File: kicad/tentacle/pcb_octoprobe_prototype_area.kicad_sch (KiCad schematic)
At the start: 15 parts, among them J1301 Conn_01x20, J1302 Conn_01x20, J1303 Conn_01x20

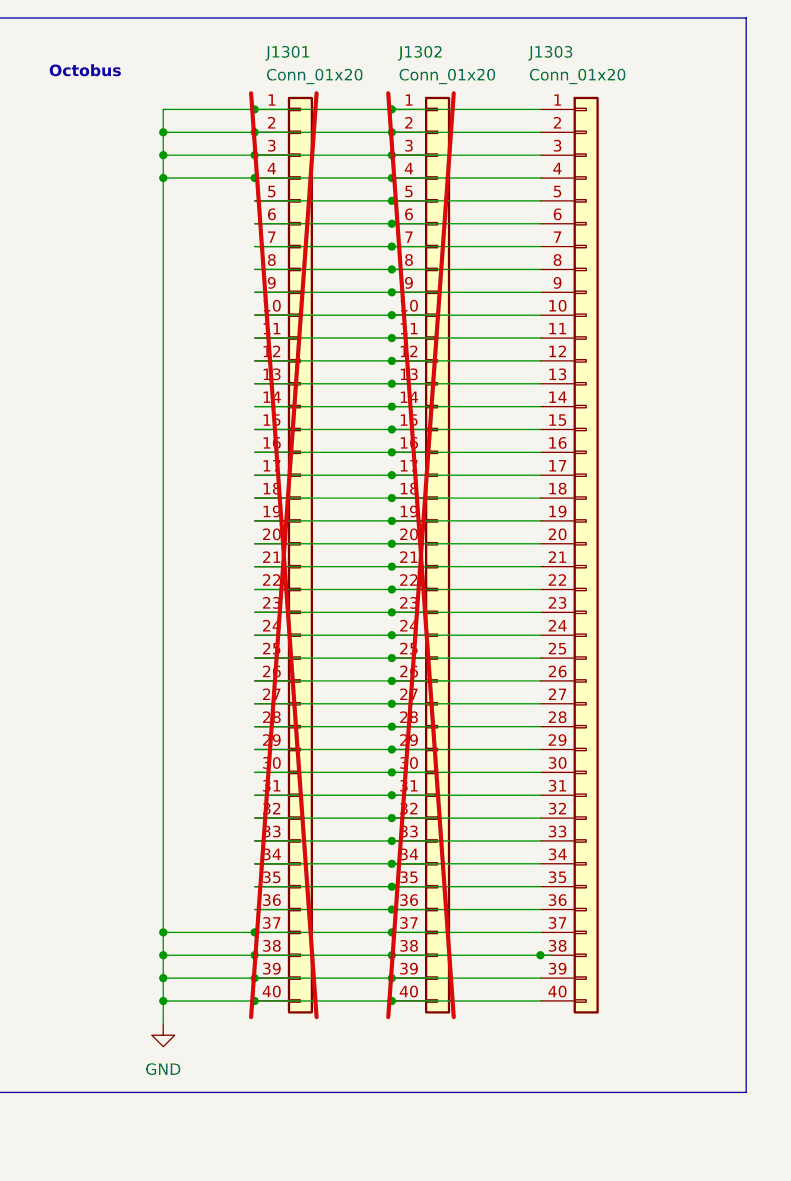
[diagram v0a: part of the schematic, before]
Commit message: Tentacle v0.4
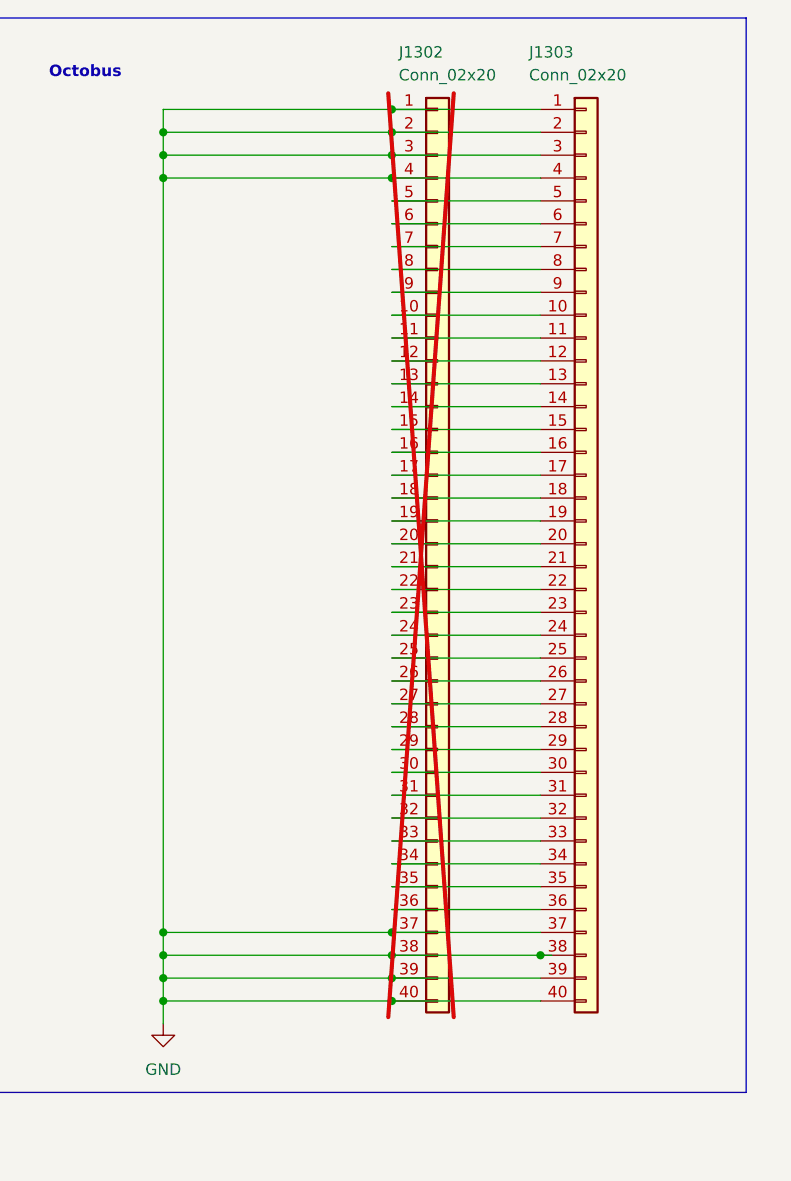
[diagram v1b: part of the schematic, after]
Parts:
- removed J1301: Conn_01x20, 00_project_library:PinSocket_2x20_P2.54mm_Vertical-stackable_squarepad, symbol Connector_Generic:Conn_01x40
- BP1301, BP1302, H1305, H1306, H1307, H1308: now left out of the parts list
- J1302, J1303: value Conn_01x20 -> Conn_02x20
